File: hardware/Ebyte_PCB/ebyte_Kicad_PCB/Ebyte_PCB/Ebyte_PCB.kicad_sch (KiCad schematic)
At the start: 18 parts, among them J1 CONMMCX001, U1 LM1085IS-12/NOPB, U10 10u, U11 10u, U12 22u, U13 121, U14 365, U15 ?, U16 ?, U2 .1u, U3 DF11, U4 TPS5405DR1, U6 4.7u, U7 22u, U8 10u, U9 85.5k

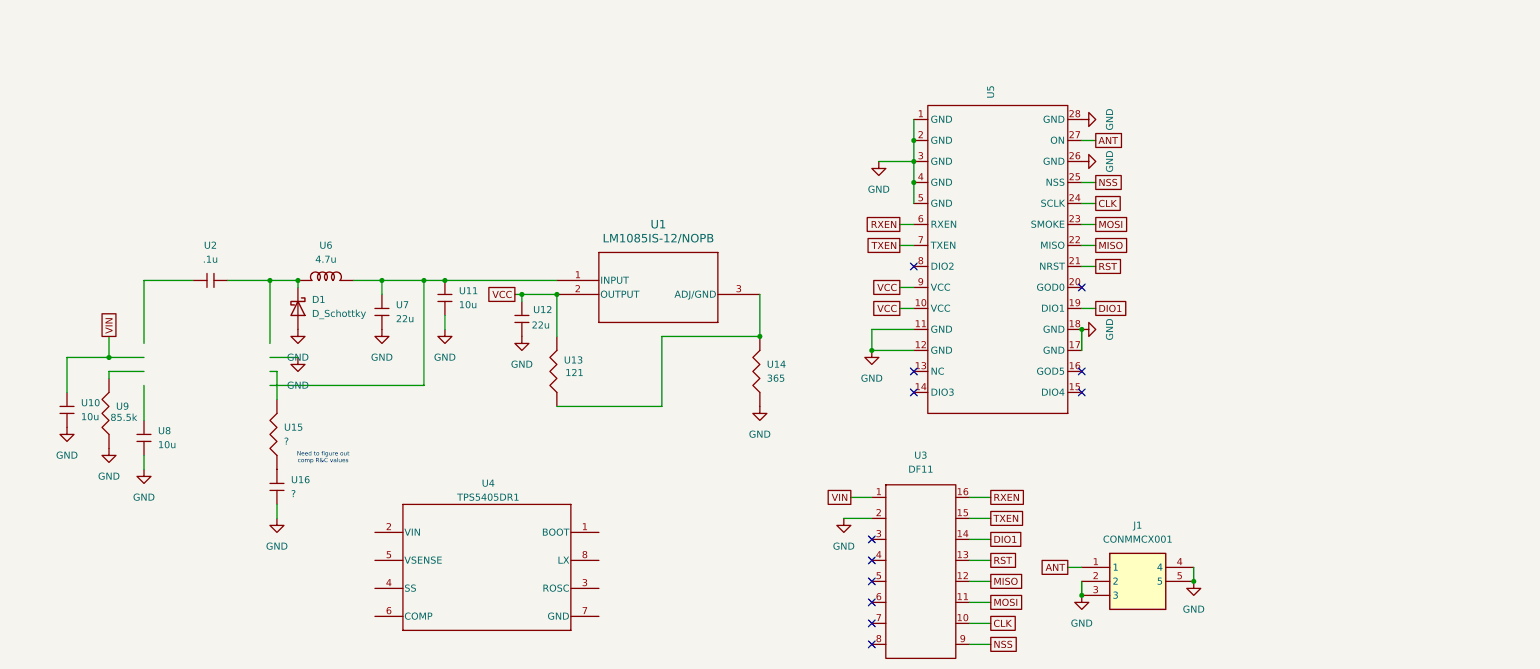
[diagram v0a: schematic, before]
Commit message: fixing schem
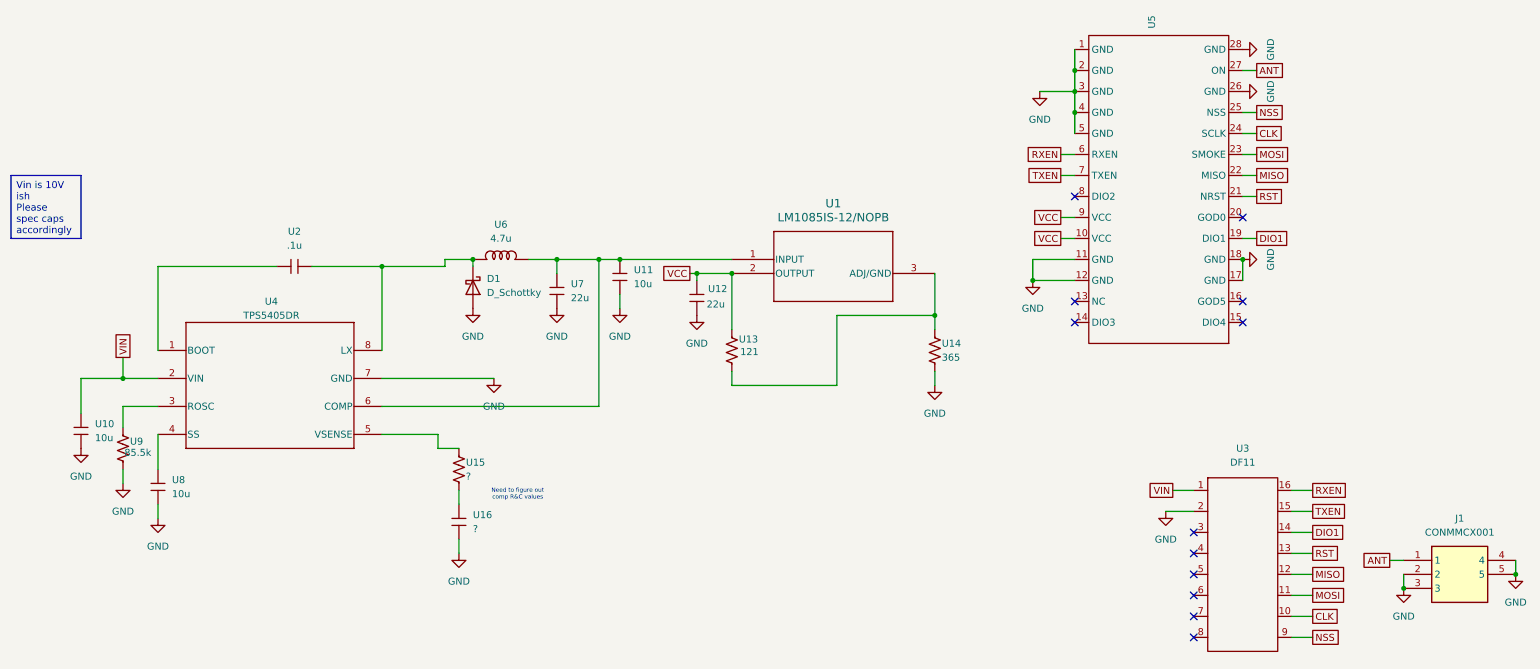
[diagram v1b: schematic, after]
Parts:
- J1: footprint ebyte_footprints:CONMMCX001 -> (none)
- U10, U11, U8: footprint (none) -> ebyte_footprints:C1206
- U4: value TPS5405DR1 -> TPS5405DR; footprint ebyte_footprints:D0008A-IPC_A -> D0008A-IPC_A
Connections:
- net GND: now also U14.~, U4.7 (GND), U9.~; no longer U14.1, U9.1
- net VCC: now also U13.~; no longer U13.2
- net VIN: now also U4.2 (VIN)
- net at U16.2: now also U15.~; no longer U15.1
- net at U8.2: now also U4.4 (SS)
- net at U2.1: now also U4.1 (BOOT)
- net at D1.1 (K), U2.2, U6.1: now also U4.8 (LX)
- net at U1.1 (INPUT), U11.2, U6.2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: now also U4.6 (COMP)
- net at U4.3 (ROSC): now also U9.~
- net at U4.5 (VSENSE): now also U15.~
- new net: U1.3 (ADJ/GND), U13.~, U14.~
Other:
- moved on the sheet: D1, J1, U1, U10, U11, U12, U16, U2, U3, U4, U5, U6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
